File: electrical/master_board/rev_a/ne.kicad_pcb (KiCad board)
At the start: 2 copper layers, 42.2 x 39 mm, 1 part, among them CN60 HCSR04;F1x4H

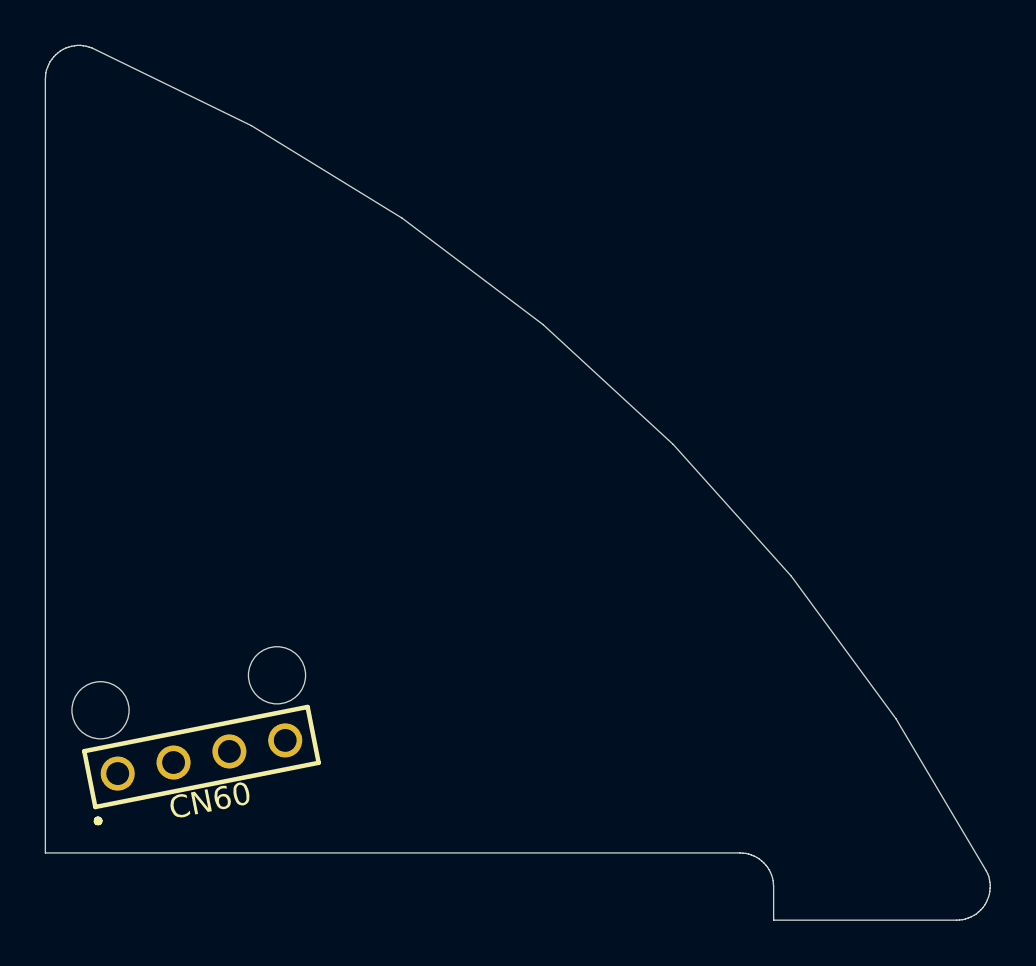
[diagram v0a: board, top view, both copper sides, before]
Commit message: Finally have everything fitting together.
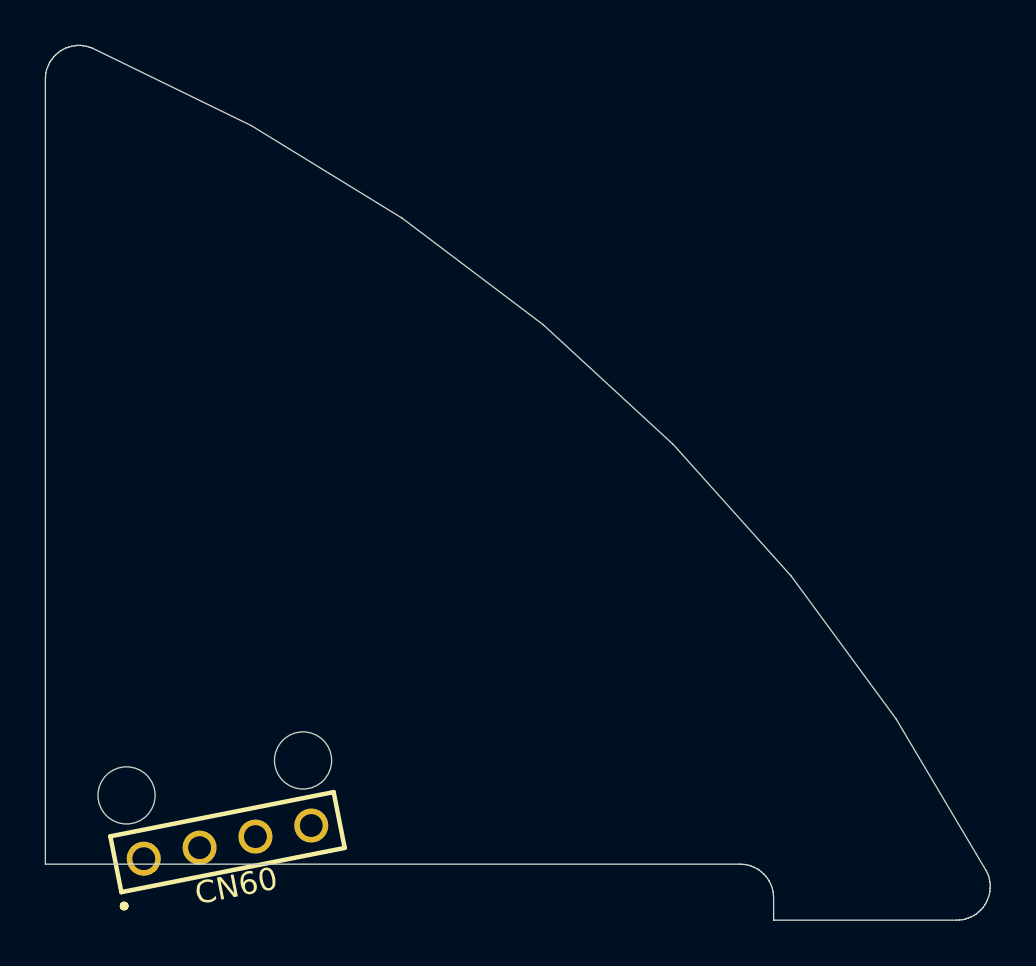
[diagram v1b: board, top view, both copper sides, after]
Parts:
- moved CN60 3.97 mm to (138.1, 60.5)
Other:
- outline, holes or cut-outs redrawn
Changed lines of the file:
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@@
   )
   (module HR2:HCSR04_F1x4H (layer F.Cu)
-    (at 136.9666 56.7177 191.2)
+    (at 138.1284 60.5169 191.2)
     (fp_text reference CN60 (at 0 -2 11.2) (layer F.SilkS)
       (effects (font (size 1 1) (thickness 0.2)))
@@
   (gr_line (start 130.02 26.19) (end 130.01 26.33) (layer Edge.Cuts) (width 0.05))
   (gr_line (start 130.01 26.33) (end 130 26.46) (layer Edge.Cuts) (width 0.05))
-  (gr_line (start 130 26.46) (end 130 61) (layer Edge.Cuts) (width 0.05))
-  (gr_line (start 130 61) (end 161 61) (layer Edge.Cuts) (width 0.05))
-  (gr_line (start 161 61) (end 161.13 61.01) (layer Edge.Cuts) (width 0.05))
-  (gr_line (start 161.13 61.01) (end 161.26 61.02) (layer Edge.Cuts) (width 0.05))
-  (gr_line (start 161.26 61.02) (end 161.39 61.05) (layer Edge.Cuts) (width 0.05))
-  (gr_line (start 161.39 61.05) (end 161.51 61.09) (layer Edge.Cuts) (width 0.05))
-  (gr_line (start 161.51 61.09) (end 161.63 61.14) (layer Edge.Cuts) (width 0.05))
-  (gr_line (start 161.63 61.14) (end 161.75 61.2) (layer Edge.Cuts) (width 0.05))
-  (gr_line (start 161.75 61.2) (end 161.86 61.27) (layer Edge.Cuts) (width 0.05))
-  (gr_line (start 161.86 61.27) (end 161.96 61.35) (layer Edge.Cuts) (width 0.05))
-  (gr_line (start 161.96 61.35) (end 162.06 61.44) (layer Edge.Cuts) (width 0.05))
-  (gr_line (start 162.06 61.44) (end 162.15 61.54) (layer Edge.Cuts) (width 0.05))
-  (gr_line (start 162.15 61.54) (end 162.23 61.64) (layer Edge.Cuts) (width 0.05))
-  (gr_line (start 162.23 61.64) (end 162.3 61.75) (layer Edge.Cuts) (width 0.05))
-  (gr_line (start 162.3 61.75) (end 162.36 61.87) (layer Edge.Cuts) (width 0.05))
-  (gr_line (start 162.36 61.87) (end 162.41 61.99) (layer Edge.Cuts) (width 0.05))
-  (gr_line (start 162.41 61.99) (end 162.45 62.11) (layer Edge.Cuts) (width 0.05))
-  (gr_line (start 162.45 62.11) (end 162.48 62.24) (layer Edge.Cuts) (width 0.05))
-  (gr_line (start 162.48 62.24) (end 162.49 62.37) (layer Edge.Cuts) (width 0.05))
-  (gr_line (start 162.49 62.37) (end 162.5 62.5) (layer Edge.Cuts) (width 0.05))
-  (gr_line (start 162.5 62.5) (end 162.5 64) (layer Edge.Cuts) (width 0.05))
+  (gr_line (start 130 26.46) (end 130 61.5) (layer Edge.Cuts) (width 0.05))
+  (gr_line (start 130 61.5) (end 161 61.5) (layer Edge.Cuts) (width 0.05))
+  (gr_line (start 161 61.5) (end 161.13 61.51) (layer Edge.Cuts) (width 0.05))
+  (gr_line (start 161.13 61.51) (end 161.26 61.52) (layer Edge.Cuts) (width 0.05))
+  (gr_line (start 161.26 61.52) (end 161.39 61.55) (layer Edge.Cuts) (width 0.05))
+  (gr_line (start 161.39 61.55) (end 161.51 61.59) (layer Edge.Cuts) (width 0.05))
+  (gr_line (start 161.51 61.59) (end 161.63 61.64) (layer Edge.Cuts) (width 0.05))
+  (gr_line (start 161.63 61.64) (end 161.75 61.7) (layer Edge.Cuts) (width 0.05))
+  (gr_line (start 161.75 61.7) (end 161.86 61.77) (layer Edge.Cuts) (width 0.05))
+  (gr_line (start 161.86 61.77) (end 161.96 61.85) (layer Edge.Cuts) (width 0.05))
+  (gr_line (start 161.96 61.85) (end 162.06 61.94) (layer Edge.Cuts) (width 0.05))
+  (gr_line (start 162.06 61.94) (end 162.15 62.04) (layer Edge.Cuts) (width 0.05))
+  (gr_line (start 162.15 62.04) (end 162.23 62.14) (layer Edge.Cuts) (width 0.05))
+  (gr_line (start 162.23 62.14) (end 162.3 62.25) (layer Edge.Cuts) (width 0.05))
+  (gr_line (start 162.3 62.25) (end 162.36 62.37) (layer Edge.Cuts) (width 0.05))
+  (gr_line (start 162.36 62.37) (end 162.41 62.49) (layer Edge.Cuts) (width 0.05))
+  (gr_line (start 162.41 62.49) (end 162.45 62.61) (layer Edge.Cuts) (width 0.05))
+  (gr_line (start 162.45 62.61) (end 162.48 62.74) (layer Edge.Cuts) (width 0.05))
+  (gr_line (start 162.48 62.74) (end 162.49 62.87) (layer Edge.Cuts) (width 0.05))
+  (gr_line (start 162.49 62.87) (end 162.5 63) (layer Edge.Cuts) (width 0.05))
+  (gr_line (start 162.5 63) (end 162.5 64) (layer Edge.Cuts) (width 0.05))
 )
